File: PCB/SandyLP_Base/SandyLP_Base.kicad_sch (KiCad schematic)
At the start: 174 parts, among them J1 Conn_01x09_Pin, J11 Conn_02x02_Odd_Even, J7 USB_C_Receptacle_USB2.0, J8 Conn_01x03, Q1 BSS138, SW1 BOOT, SW2 RESET, U1 NCP1117-3.3_SOT223, U2 RP2040, U3 W25Q128JVPIQ, Y1 12MHz

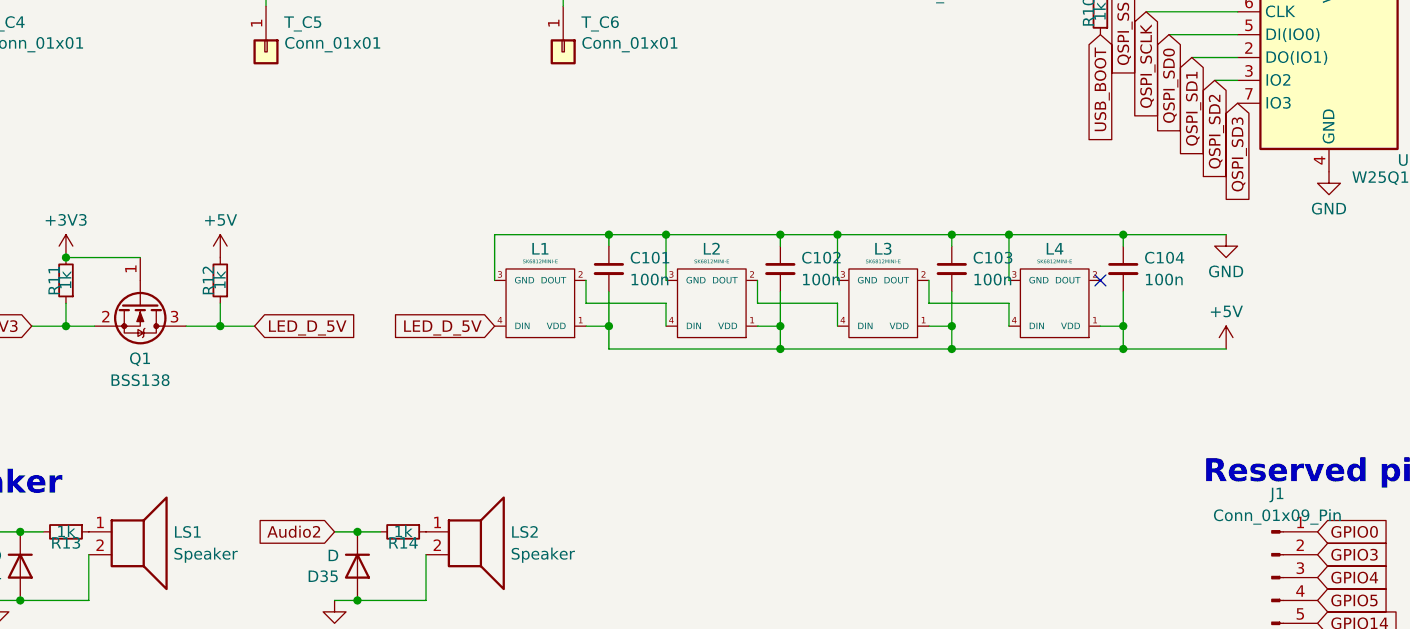
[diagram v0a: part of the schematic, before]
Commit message: WIP パーツ配置
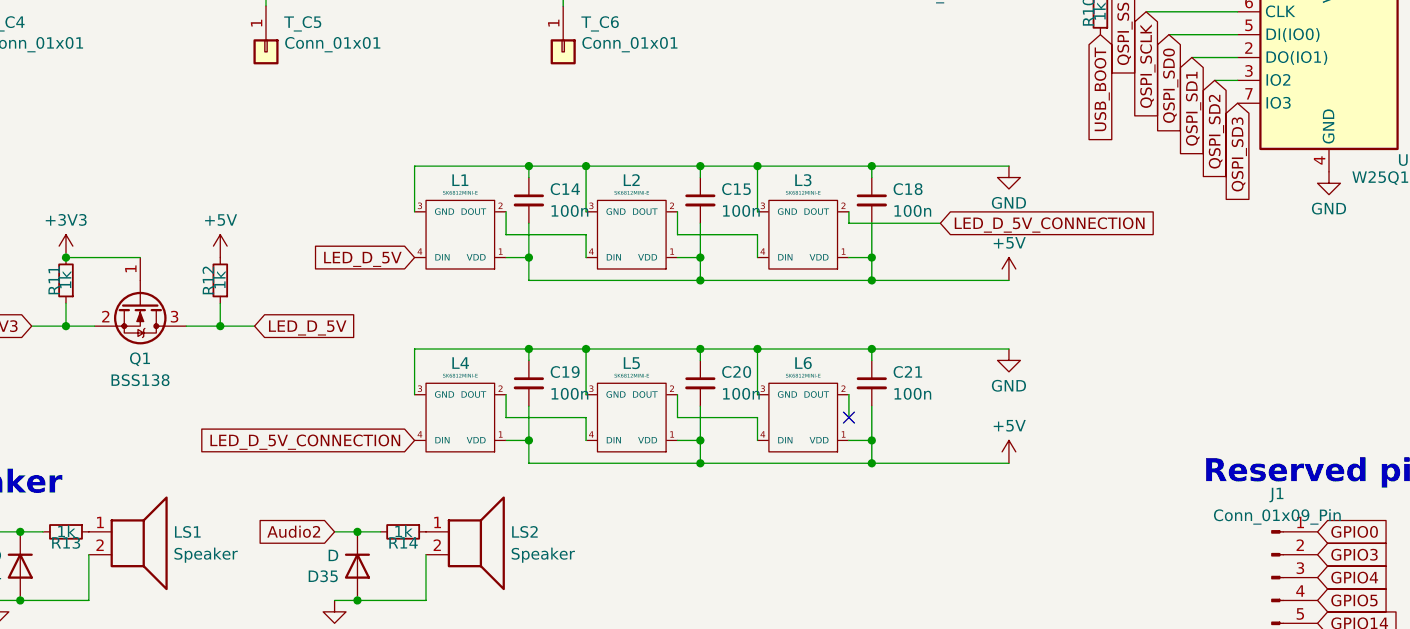
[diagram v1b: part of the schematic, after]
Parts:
- removed C101, C102, C103, C104: 100n, Capacitor_SMD:C_0402_1005Metric, symbol Device:C_Small
- added C14, C15, C18, C19, C20, C21: 100n, Capacitor_SMD:C_0402_1005Metric, symbol Device:C_Small
- added L5, L6: SK6812MINI-E, locallib:YS-SK6812MINI-E_middle_hole_with_small_pad, symbol kbd:SK6812MINI-E
- J1: footprint (none) -> Connector_PinHeader_1.00mm:PinHeader_1x09_P1.00mm_Vertical
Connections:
- net +5V: now also C14.2, C15.2, C18.2, C19.2, C20.2, C21.2, L5.1 (VDD), L6.1 (VDD)
- net GND: now also C14.1, C15.1, C18.1, C19.1, C20.1, C21.1, L5.3 (GND), L6.3 (GND)
- net LED_D_5V_CONNECTION: now reaches L3.2 (DOUT), L4.4 (DIN)
- net at L4.2 (DOUT): now also L5.4 (DIN)
- new net: L5.2 (DOUT), L6.4 (DIN)
